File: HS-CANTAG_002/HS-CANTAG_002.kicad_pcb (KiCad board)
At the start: 2 copper layers, 100 x 60 mm, 27 parts, among them J1 5v_GND, J2 CAN_SPI, J3 AudioJack, J4 Debug_Serial, J5 Serial_5v, J6 i2c_3.3v, SW1 ID_DIP, U1 AE-ATMEGA328-MINI, U2 DFPLAYER_MINI, U3 R-783.3-0.5, U4 TWELITE_DIP

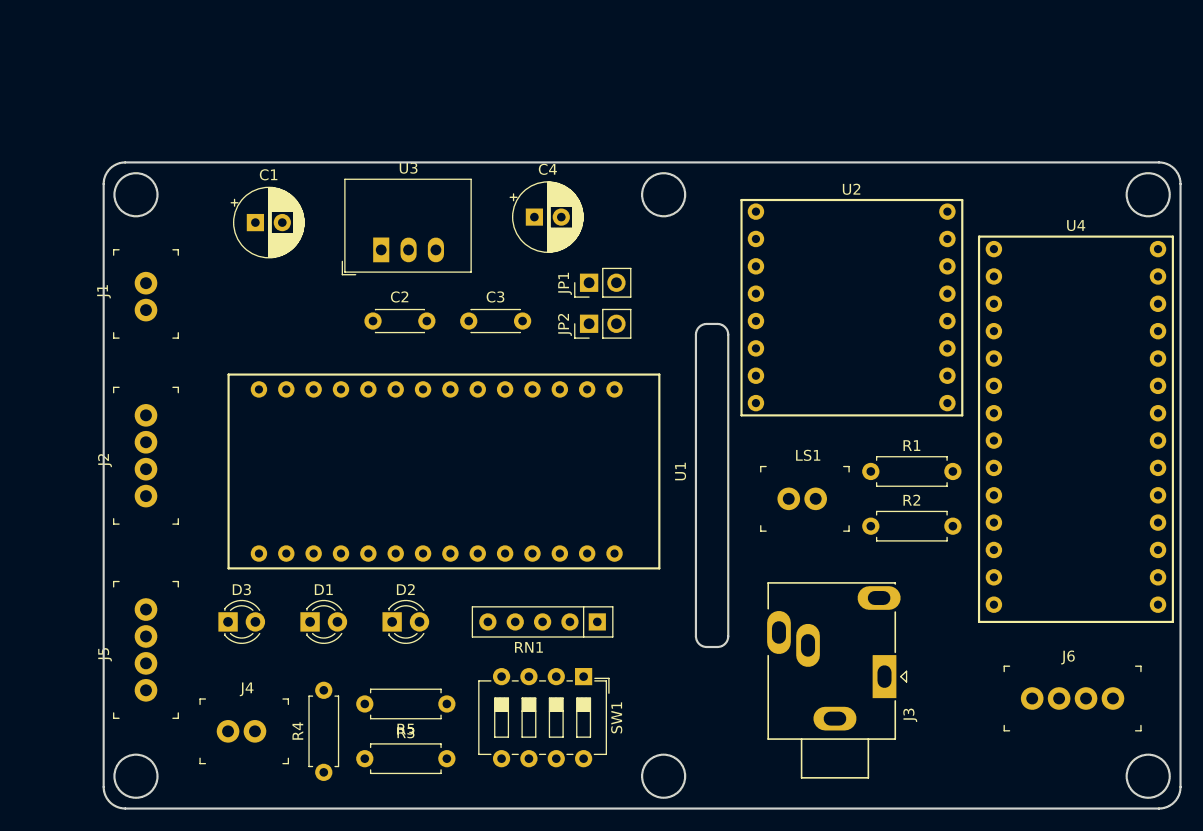
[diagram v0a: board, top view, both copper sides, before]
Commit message: ・CANTAG_002基盤概成
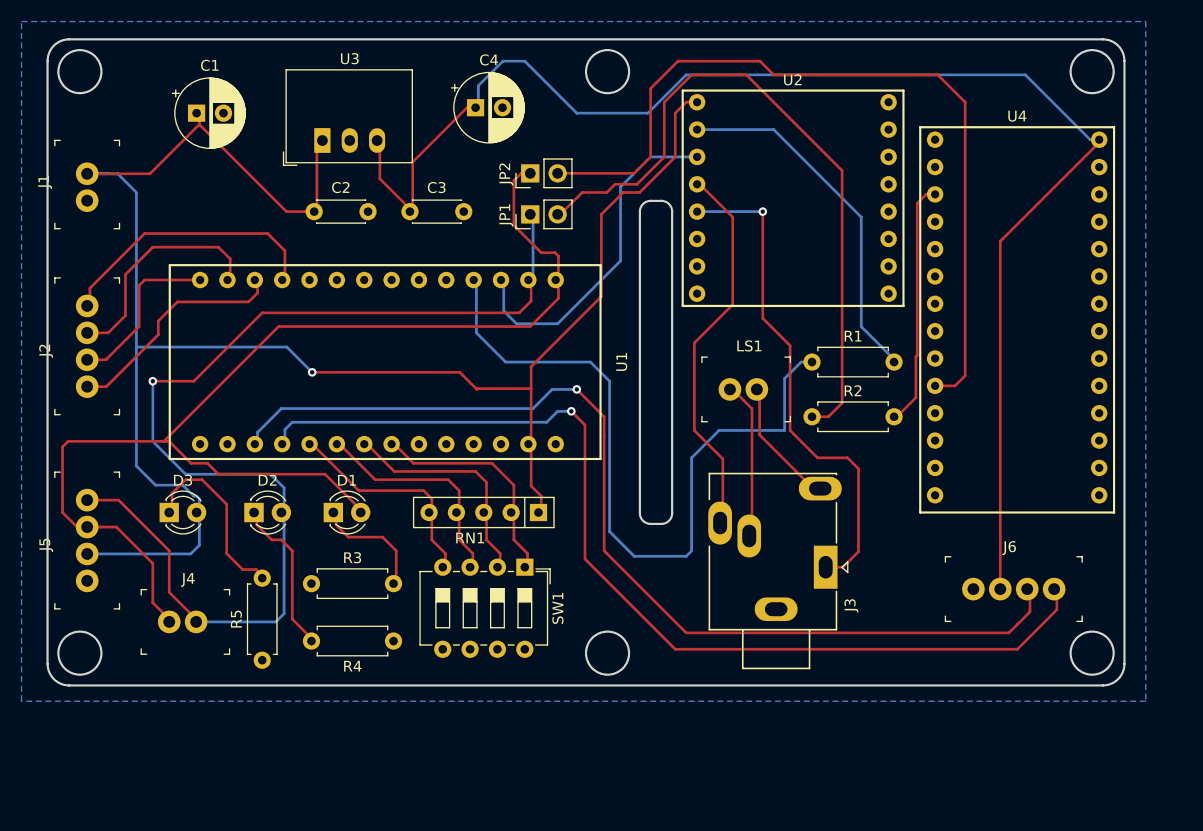
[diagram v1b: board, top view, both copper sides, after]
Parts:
- moved R5 17.6 mm to (109.9, 110.2), turned to 90 degrees
- moved R3 17.0 mm to (114.4, 103.1)
- moved D2 16.4 mm to (109.1, 96.5)
- moved JP2 15.0 mm to (134.7, 65.0)
- moved R4 13.8 mm to (122.0, 108.5), turned to 180 degrees
- moved D3 11.5 mm to (101.2, 96.5)
- moved R2 11.5 mm to (160.9, 87.6)
- moved RN1 11.5 mm to (135.5, 96.5)
- moved J1 11.5 mm to (93.6, 67.6)
- moved C3 11.5 mm to (123.6, 68.6)
- moved J4 11.5 mm to (101.2, 106.7)
- moved LS1 11.5 mm to (153.3, 85.1)
- moved R1 11.5 mm to (160.9, 82.5)
- moved U2 11.5 mm to (159.1, 67.3)
- moved C1 11.5 mm to (103.8, 59.4)
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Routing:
- net +5V: track 0.00 -> 173.5 mm, vias 0 -> 1
- net +3.3V: track 0.00 -> 133.2 mm
- net RX_H: track 0.00 -> 111.1 mm
- net TX_H: track 0.00 -> 102.9 mm, vias 0 -> 1
- net SCL: track 0.00 -> 94.0 mm, vias 0 -> 1
- net SDA: track 0.00 -> 93.6 mm, vias 0 -> 1
- net Net-(JP2-Pad2): track 0.00 -> 75.5 mm
- net Net-(R1-Pad1): track 0.00 -> 68.5 mm
- net Net-(JP1-Pad2): track 0.00 -> 62.8 mm
- net Net-(J3-PadT): track 0.00 -> 46.1 mm, vias 0 -> 1
- net Net-(J3-PadR): track 0.00 -> 35.3 mm
- net Net-(R1-Pad2): track 0.00 -> 33.2 mm
- net Net-(U1-Pad3): track 0.00 -> 32.0 mm
- net CS: track 0.00 -> 25.2 mm
- net Net-(R2-Pad2): track 0.00 -> 22.9 mm
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- added copper zone on B.Cu, net GND
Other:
- board text added: "HS-CANTAG_002"
